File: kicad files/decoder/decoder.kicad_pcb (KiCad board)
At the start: 2 copper layers, 102.9 x 49.5 mm, 8 parts

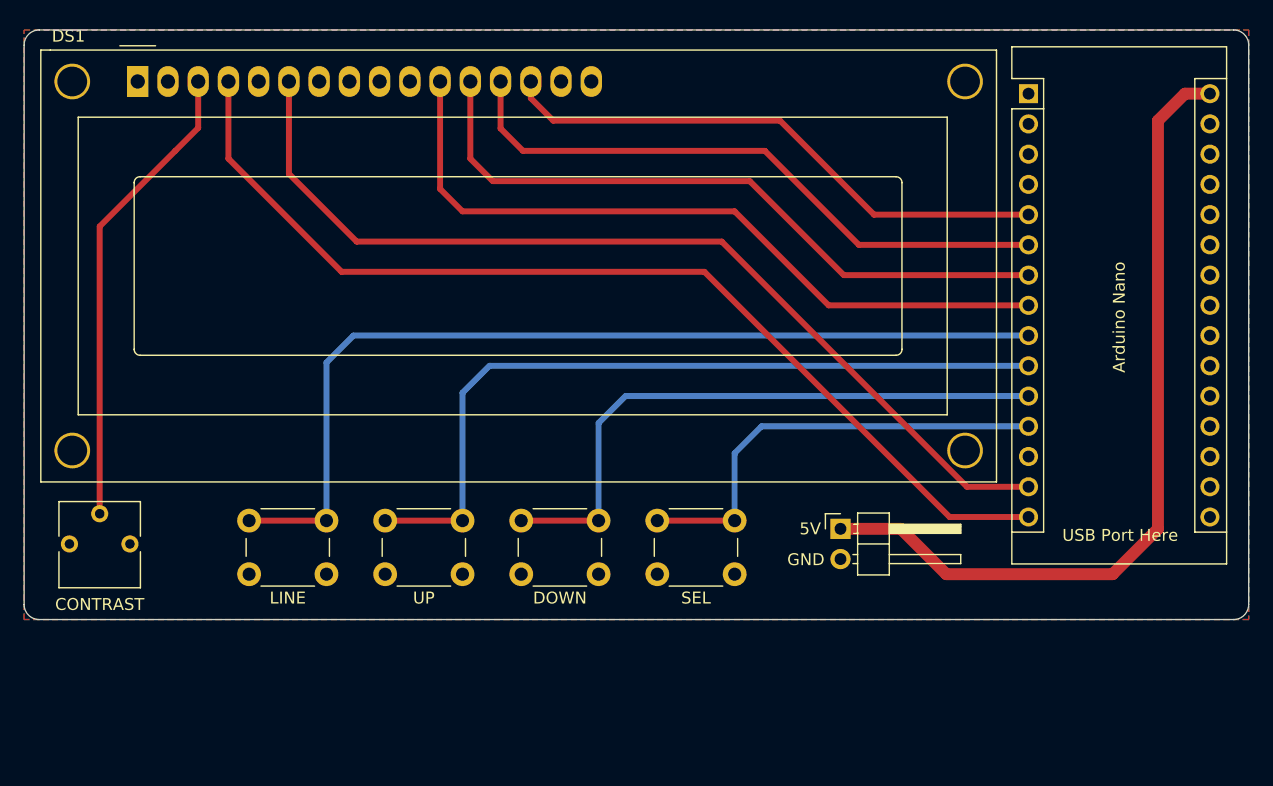
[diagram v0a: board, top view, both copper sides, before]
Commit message: final changes to PCB, started to clean up code on first gen PCB
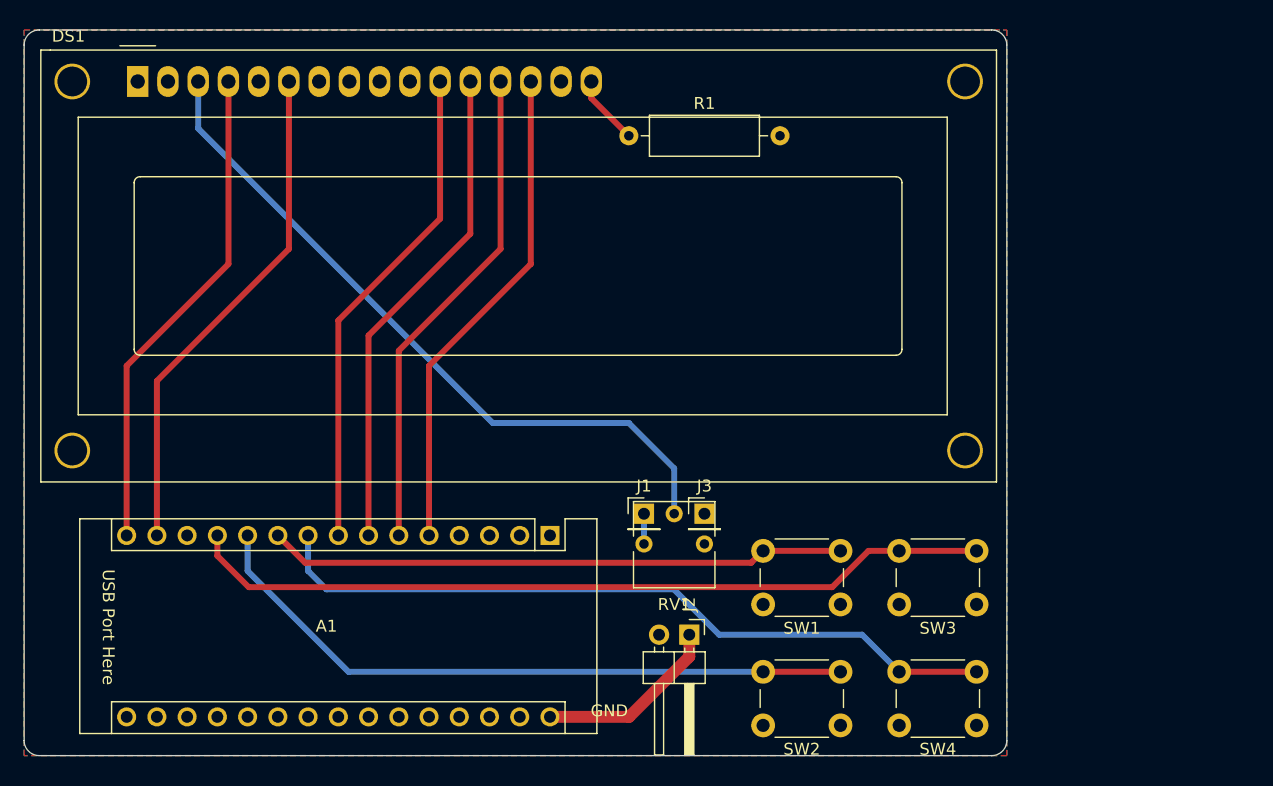
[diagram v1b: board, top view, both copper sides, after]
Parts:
- added J1: Conn_01x01_Male, Connector_PinHeader_2.54mm:PinHeader_1x01_P2.54mm_Vertical, F.Cu at (125.7, 102.9)
- added J3: Conn_01x01_Male, Connector_PinHeader_2.54mm:PinHeader_1x01_P2.54mm_Vertical, F.Cu at (130.8, 102.9)
- added R1: 220, Resistor_THT:R_Axial_DIN0309_L9.0mm_D3.2mm_P12.70mm_Horizontal, F.Cu at (124.5, 71.1)
- A1: renamed from Arduino Nano
- moved SW4 56.1 mm to (153.7, 120.7)
- moved A1 54.7 mm to (117.8, 104.7), turned to 270 degrees
- moved RV1 48.3 mm to (130.8, 105.4)
- moved SW1 31.9 mm to (142.2, 110.5)
- moved SW2 24.0 mm to (142.2, 120.7)
- moved SW3 20.5 mm to (153.7, 110.5)
- moved J2 15.5 mm to (129.5, 113.0), turned to 270 degrees
- renumbered 5V to J2, CONTRAST to RV1, UP to SW1, DOWN to SW2, SEL to SW3, LINE to SW4
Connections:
- DS1 pad 16: GND -> Net-(DS1-Pad16)
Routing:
- net VIN: track 69.4 -> 15.6 mm
- net RS: track 86.2 -> 41.7 mm
- net Enable: track 80.8 -> 42.7 mm
- net Net-(A1-Pad12): track 37.8 -> 67.8 mm
- net D4: track 62.5 -> 41.7 mm
- net Contrast: track 39.7 -> 59.6 mm
- net Net-(A1-Pad10): track 65.7 -> 48.6 mm
- net Net-(A1-Pad9): track 79.7 -> 62.6 mm
- net D5: track 57.4 -> 41.7 mm
- net D6: track 52.3 -> 41.7 mm
- net Net-(DS1-Pad16): track 0.00 -> 5.87 mm
- net D7: track 47.3 -> 41.7 mm
- net Net-(A1-Pad11): track 51.8 -> 56.3 mm
- net +5V: track 0.00 -> 2.54 mm
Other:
- board size 102.9 x 49.5 mm -> 82.6 x 61 mm
